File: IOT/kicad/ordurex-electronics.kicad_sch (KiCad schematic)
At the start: 1 part

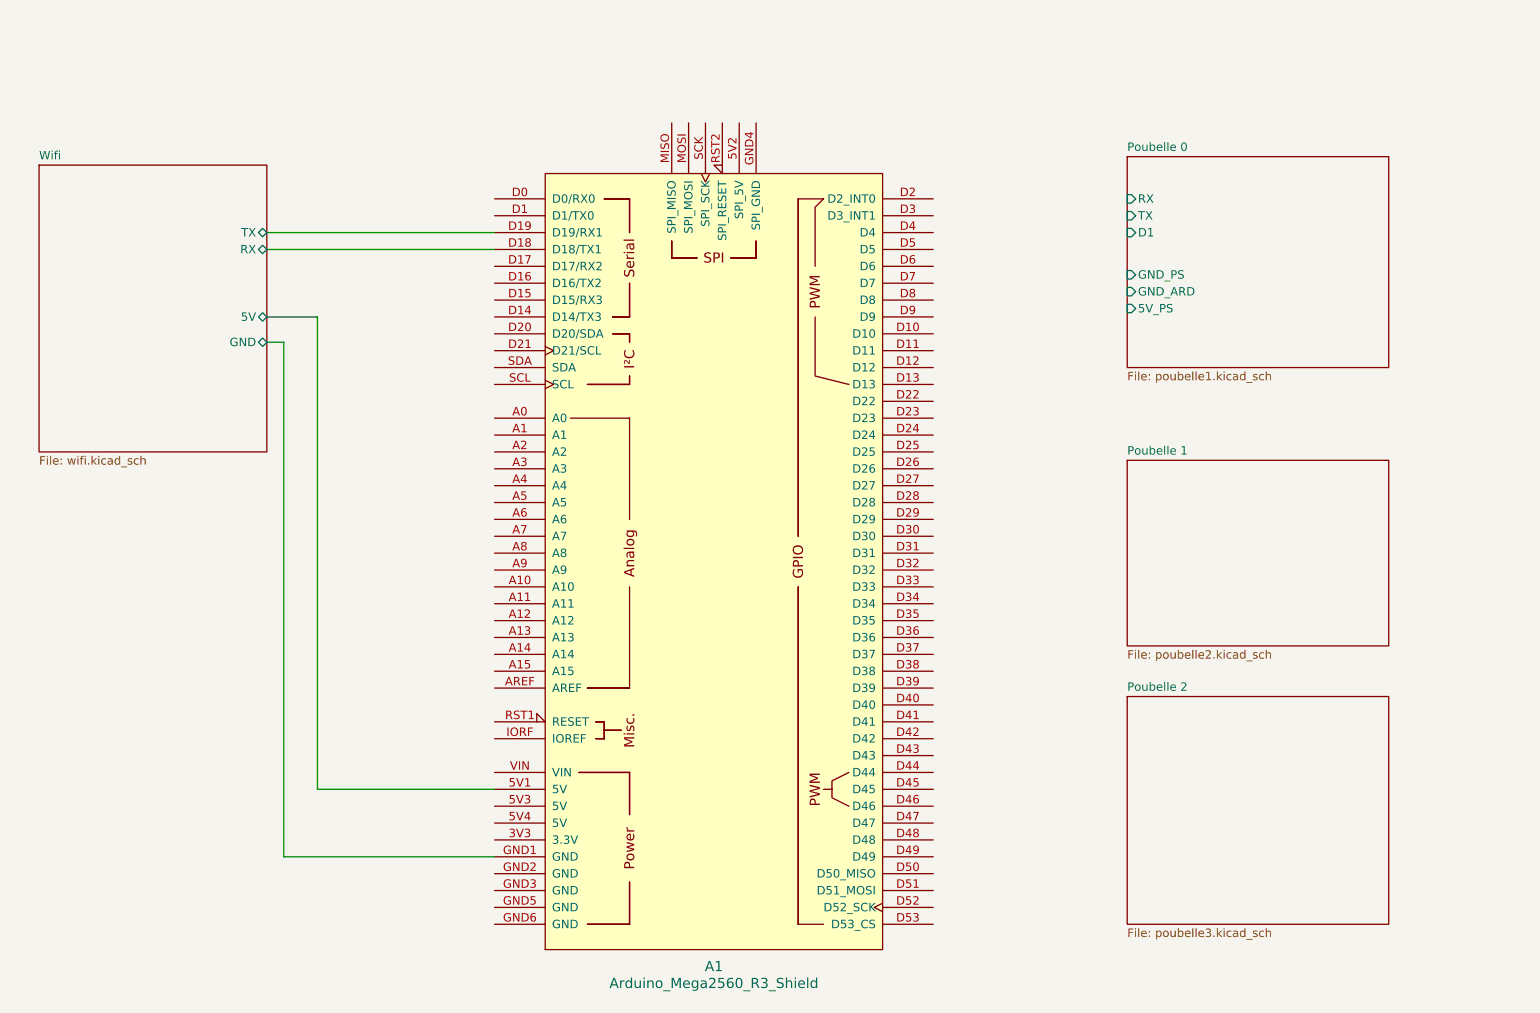
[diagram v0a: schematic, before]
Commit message: docs(iot): kicad pbl0 pbl1
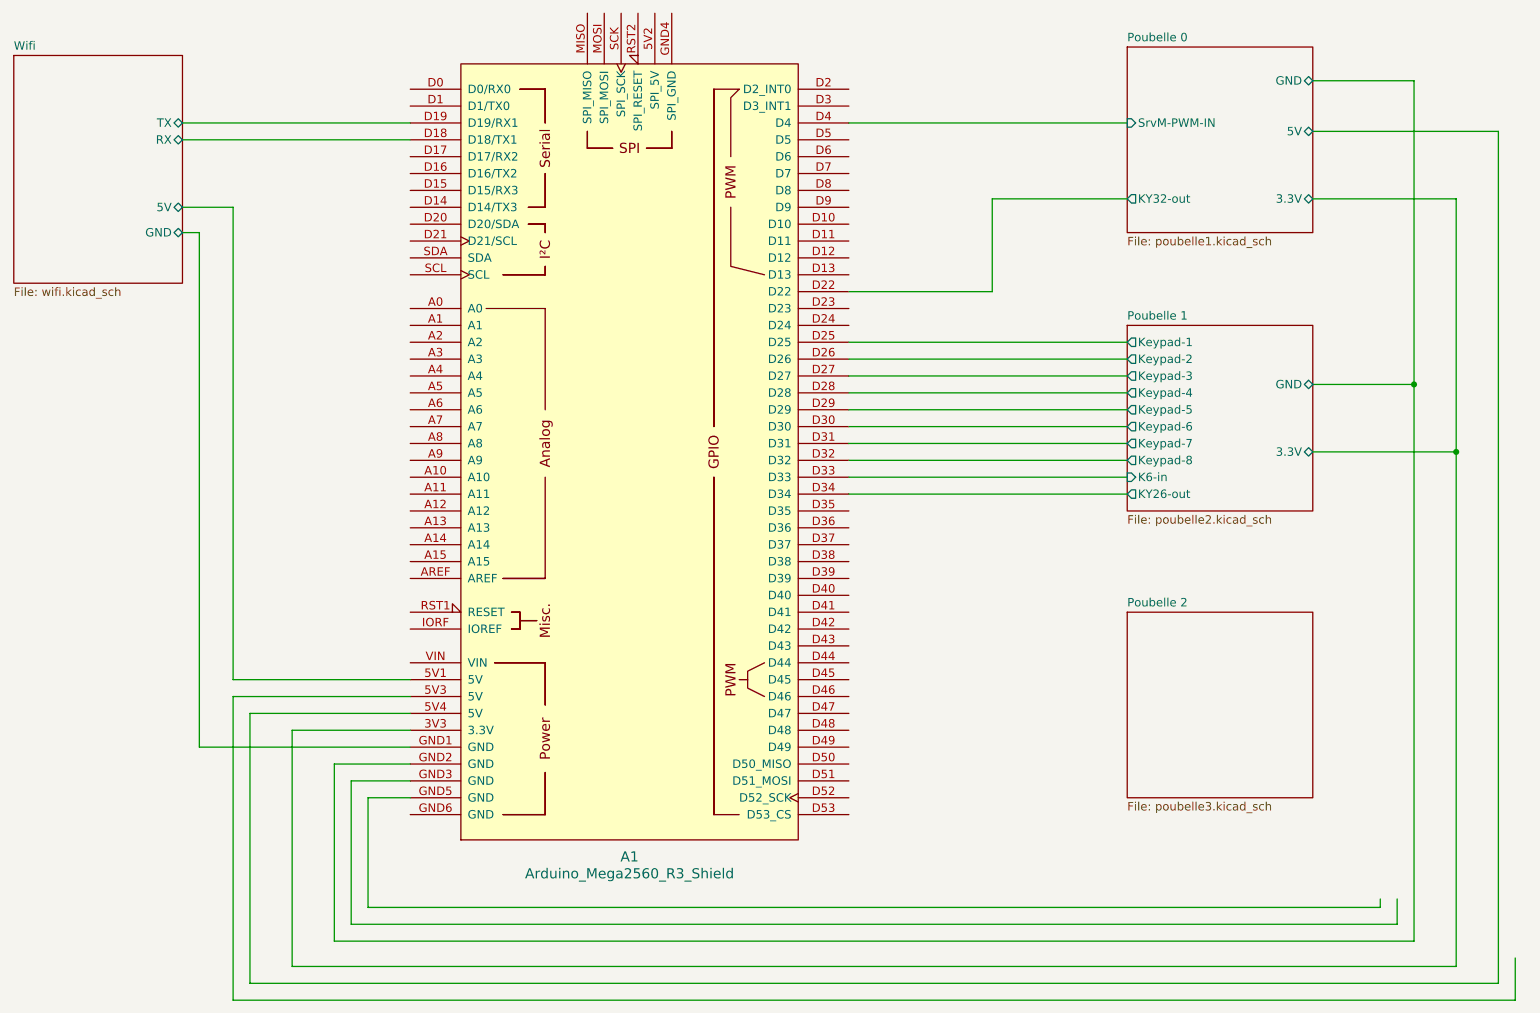
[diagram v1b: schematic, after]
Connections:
- net Poubelle 0/3.3V: now reaches A1.3V3 (3.3V)
- net Poubelle 0/5V: now reaches A1.5V4 (5V)
- net Poubelle 0/KY32-out: now reaches A1.D22
- net Poubelle 1/Keypad-1: now reaches A1.D25
- net Poubelle 1/Keypad-2: now reaches A1.D26
- net Poubelle 1/Keypad-3: now reaches A1.D27
- net Poubelle 1/Keypad-4: now reaches A1.D28
- net Poubelle 1/Keypad-5: now reaches A1.D29
- net Poubelle 1/Keypad-6: now reaches A1.D30
- net Poubelle 1/Keypad-7: now reaches A1.D31
- net Poubelle 1/Keypad-8: now reaches A1.D32
- net Poubelle 1/K6-in: now reaches A1.D33
- net Poubelle 1/KY26-out: now reaches A1.D34
- net Poubelle 0/SrvM-PWM-IN: now reaches A1.D4
- net Poubelle 0/GND: now reaches A1.GND2 (GND)
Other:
- sheet Poubelle 0 ports: added 3.3V, 5V, GND, KY32-out, SrvM-PWM-IN; removed 5V_PS, D1, GND_ARD, GND_PS, RX, TX
- sheet Poubelle 1 ports: added 3.3V, GND, K6-in, KY26-out, Keypad-1, Keypad-2, Keypad-3, Keypad-4, Keypad-5, Keypad-6, Keypad-7, Keypad-8; removed none
- moved on the sheet: A1

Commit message: docs(iot): pbl 1 & 2
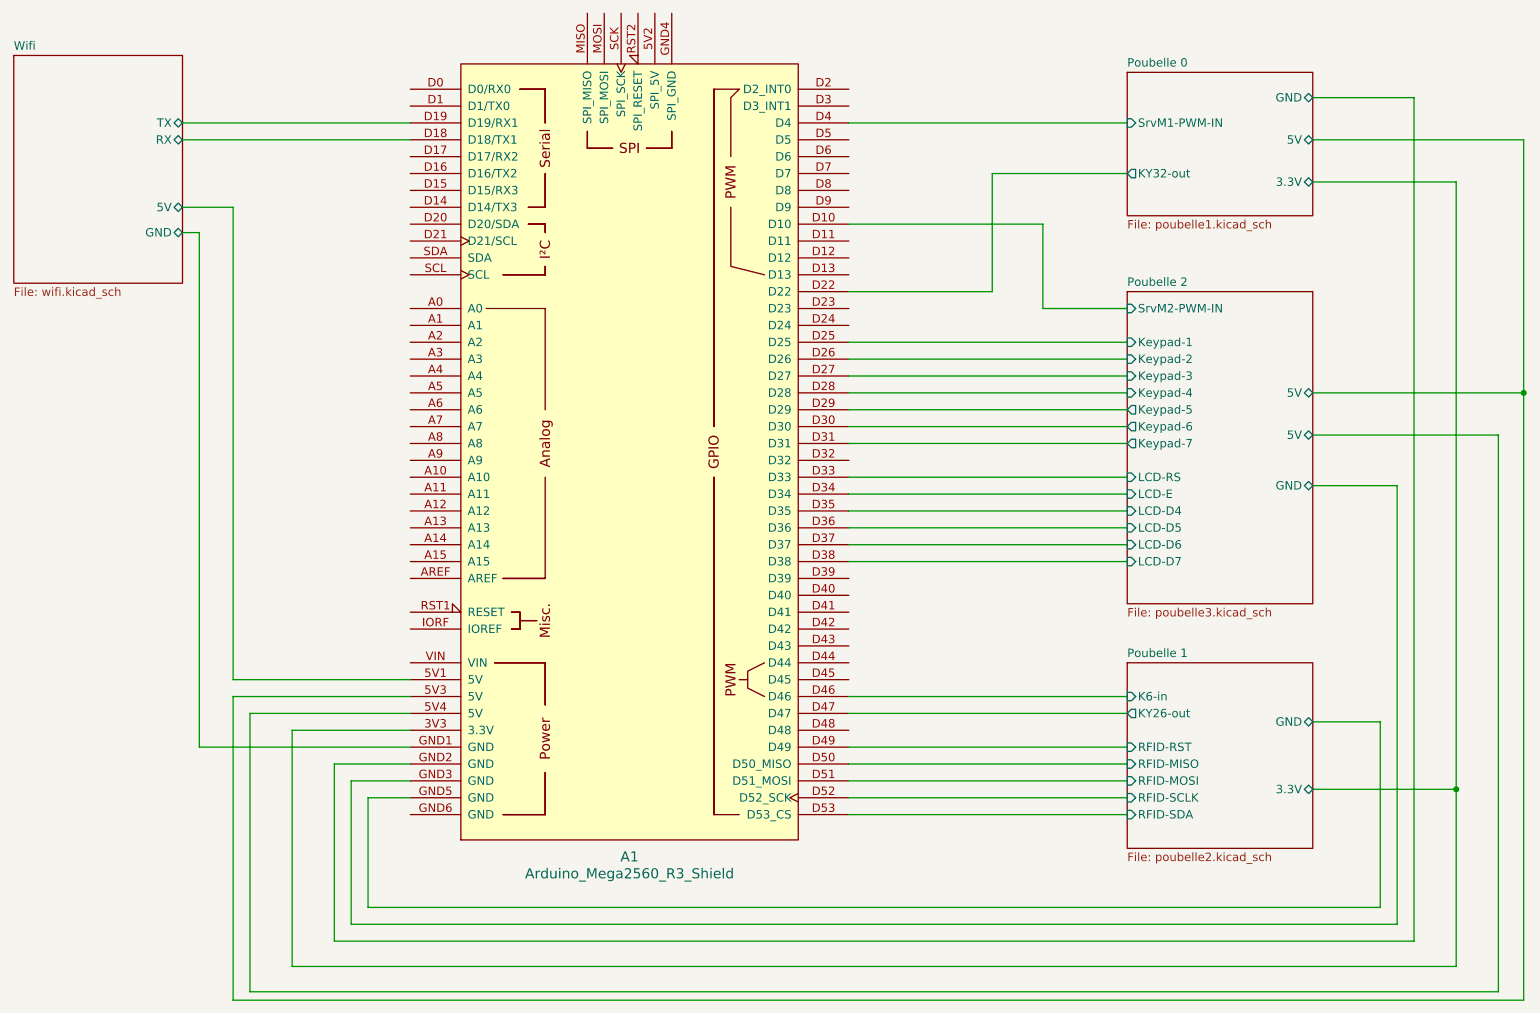
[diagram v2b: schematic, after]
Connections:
- net Poubelle 0/5V: now also A1.5V3 (5V); no longer A1.5V4 (5V)
- net Poubelle 1/K6-in: now also A1.D46; no longer A1.D33
- net Poubelle 1/KY26-out: now also A1.D47; no longer A1.D34
- net Poubelle 2/SrvM2-PWM-IN: now reaches A1.D10
- net Poubelle 2/LCD-D4: now reaches A1.D35
- net Poubelle 2/LCD-D5: now reaches A1.D36
- net Poubelle 2/LCD-D6: now reaches A1.D37
- net Poubelle 2/LCD-D7: now reaches A1.D38
- net Poubelle 1/RFID-RST: now reaches A1.D49
- net Poubelle 1/RFID-MISO: now reaches A1.D50 (D50_MISO)
- net Poubelle 1/RFID-MOSI: now reaches A1.D51 (D51_MOSI)
- net Poubelle 1/RFID-SCLK: now reaches A1.D52 (D52_SCK)
- net Poubelle 1/RFID-SDA: now reaches A1.D53 (D53_CS)
- net Poubelle 2/GND: now reaches A1.GND3 (GND)
- net Poubelle 1/GND: now reaches A1.GND5 (GND)
- net Poubelle 0/SrvM-PWM-IN renamed Poubelle 0/SrvM1-PWM-IN
- net Poubelle 1/Keypad-1 renamed Poubelle 2/Keypad-1
- net Poubelle 1/Keypad-2 renamed Poubelle 2/Keypad-2
- net Poubelle 1/Keypad-3 renamed Poubelle 2/Keypad-3
- net Poubelle 1/Keypad-4 renamed Poubelle 2/Keypad-4
- net Poubelle 1/Keypad-5 renamed Poubelle 2/Keypad-5
- net Poubelle 1/Keypad-6 renamed Poubelle 2/Keypad-6
- net Poubelle 1/Keypad-7 renamed Poubelle 2/Keypad-7
- net Poubelle 1/Keypad-8: no longer names the net of A1.D32
- new net Poubelle 2/5V: A1.5V4 (5V)
- new net Poubelle 2/LCD-E: A1.D34
- new net Poubelle 2/LCD-RS: A1.D33
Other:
- sheet Poubelle 0 ports: added SrvM1-PWM-IN; removed SrvM-PWM-IN
- sheet Poubelle 1 ports: added RFID-MISO, RFID-MOSI, RFID-RST, RFID-SCLK, RFID-SDA; removed Keypad-1, Keypad-2, Keypad-3, Keypad-4, Keypad-5, Keypad-6, Keypad-7, Keypad-8
- sheet Poubelle 2 ports: added 5V, GND, Keypad-1, Keypad-2, Keypad-3, Keypad-4, Keypad-5, Keypad-6, Keypad-7, LCD-D4, LCD-D5, LCD-D6, LCD-D7, LCD-E, LCD-RS, SrvM2-PWM-IN; removed none
